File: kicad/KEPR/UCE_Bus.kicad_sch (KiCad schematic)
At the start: 2 parts, among them J1 SODIMM-200, J2 SODIMM-200

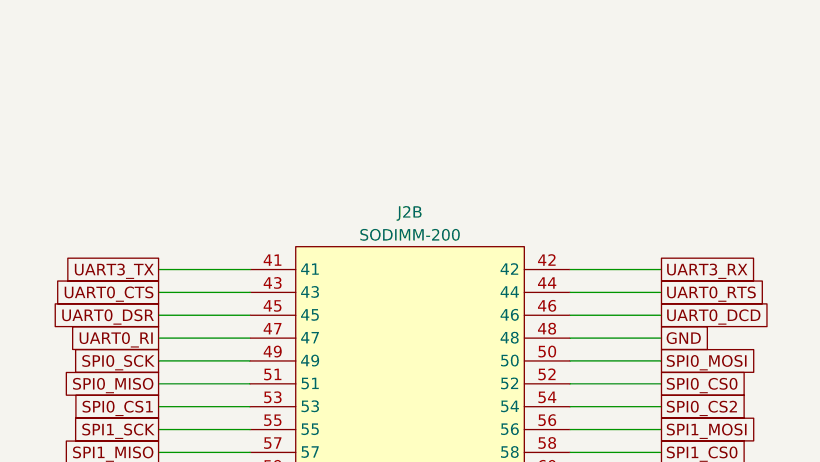
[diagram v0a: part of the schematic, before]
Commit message: Iniciado projeto da PCB, para uma referência de tamanho.
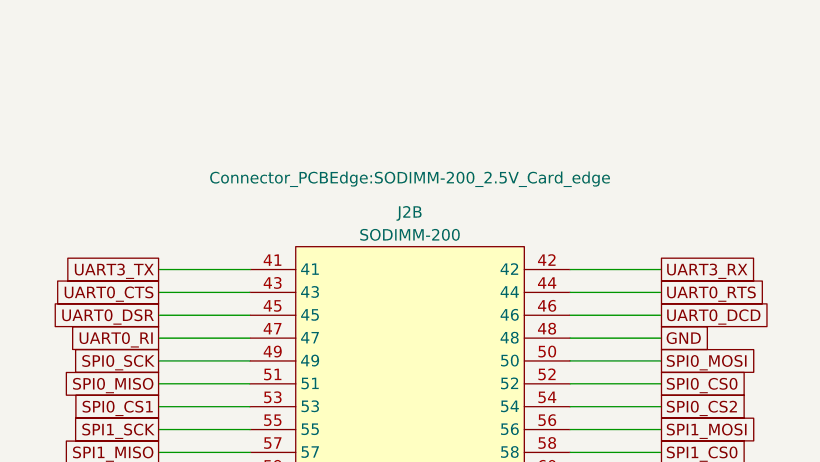
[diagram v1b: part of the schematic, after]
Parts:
- J2: footprint (none) -> Connector_PCBEdge:SODIMM-200_2.5V_Card_edge
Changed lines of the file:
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@@
 					(size 1.27 1.27)
 				)
-				(hide yes)
 			)
 		)
@@
 		(on_board yes)
 		(dnp no)
-		(fields_autoplaced yes)
 		(property "Reference" "J2"
 			(at 167.64 41.91 0)
@@
 			)
 		)
-		(property "Footprint" ""
-			(at 203.2 49.53 0)
+		(property "Footprint" "Connector_PCBEdge:SODIMM-200_2.5V_Card_edge"
+			(at 167.64 38.1 0)
 			(effects
 				(font
 					(size 1.27 1.27)
 				)
-				(hide yes)
-			)
-		)
+			)
+		)
